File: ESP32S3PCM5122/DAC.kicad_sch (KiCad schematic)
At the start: 17 parts, among them J1 OUT, U2 PCM5242, U3 OPA1656

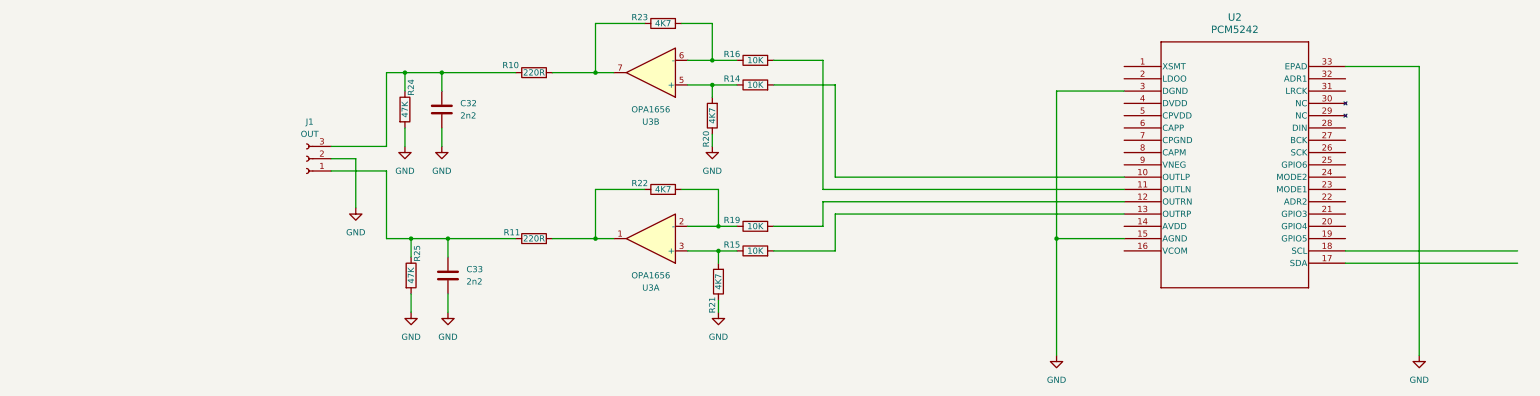
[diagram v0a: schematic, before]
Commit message: more work
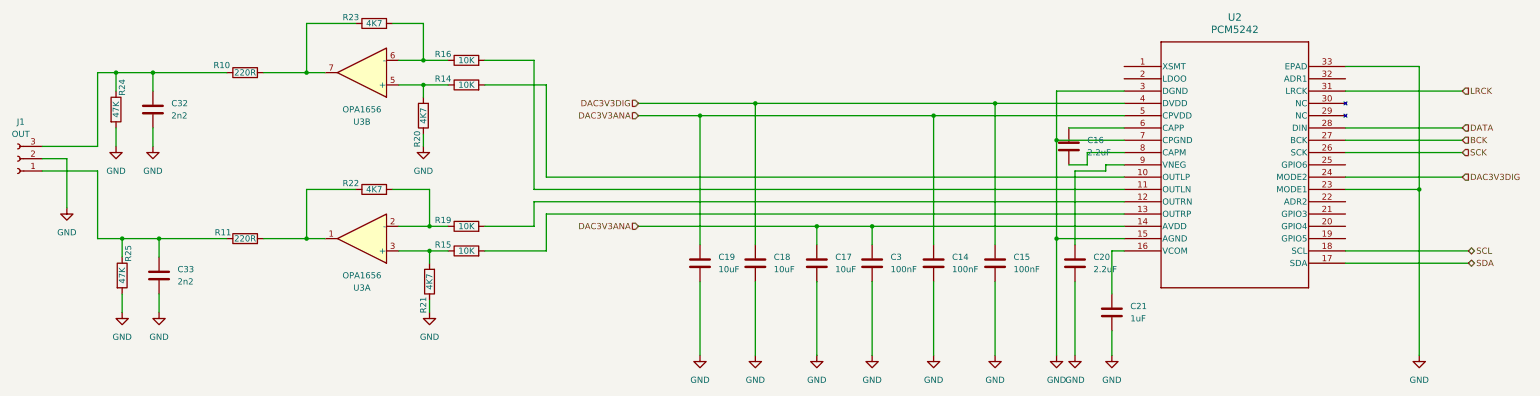
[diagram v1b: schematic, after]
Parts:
- added C14, C15, C3: 100nF, Capacitor_SMD:C_1206_3216Metric_Pad1.33x1.80mm_HandSolder, symbol Device:C
- added C16, C20: 2.2uF, Capacitor_SMD:C_0805_2012Metric_Pad1.18x1.45mm_HandSolder, symbol Device:C
- added C17, C18, C19: 10uF, Capacitor_SMD:C_0805_2012Metric_Pad1.18x1.45mm_HandSolder, symbol Device:C
- added C21: 1uF, Capacitor_SMD:C_1206_3216Metric_Pad1.33x1.80mm_HandSolder, symbol Device:C
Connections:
- net GND: now also U2.23 (MODE1), U2.7 (CPGND), C14.2, C15.2, C17.2, C18.2, C19.2, C20.2, C21.2, C3.2
- net DAC3V3ANA: now reaches U2.14 (AVDD)
- net DAC3V3ANA: now also U2.5 (CPVDD), C14.1, C17.1, C19.1, C3.1
- net at U2.16 (VCOM): now also C21.1
- net SDA: now reaches U2.17 (SDA)
- net SCL: now reaches U2.18 (SCL)
- net DAC3V3DIG: now reaches U2.24 (MODE2)
- net DAC3V3DIG: now also U2.4 (DVDD), C15.1, C18.1
- net SCK: now reaches U2.26 (SCK)
- net BCK: now reaches U2.27 (BCK)
- net DATA: now reaches U2.28 (DIN)
- net LRCK: now reaches U2.31 (LRCK)
- net at U2.6 (CAPP): now also C16.1
- net at U2.8 (CAPM): now also C16.2
- net at U2.9 (VNEG): now also C20.1
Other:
- moved on the sheet: C32, C33, J1, R10, R11, R14, R15, R16, R19, R20, R21, R22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
